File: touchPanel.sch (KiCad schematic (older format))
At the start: 41 parts, among them U11 MCP1703, U12 QT1481, U14 AFX-01_BUTTON_MATRIX, X2 16Mhz

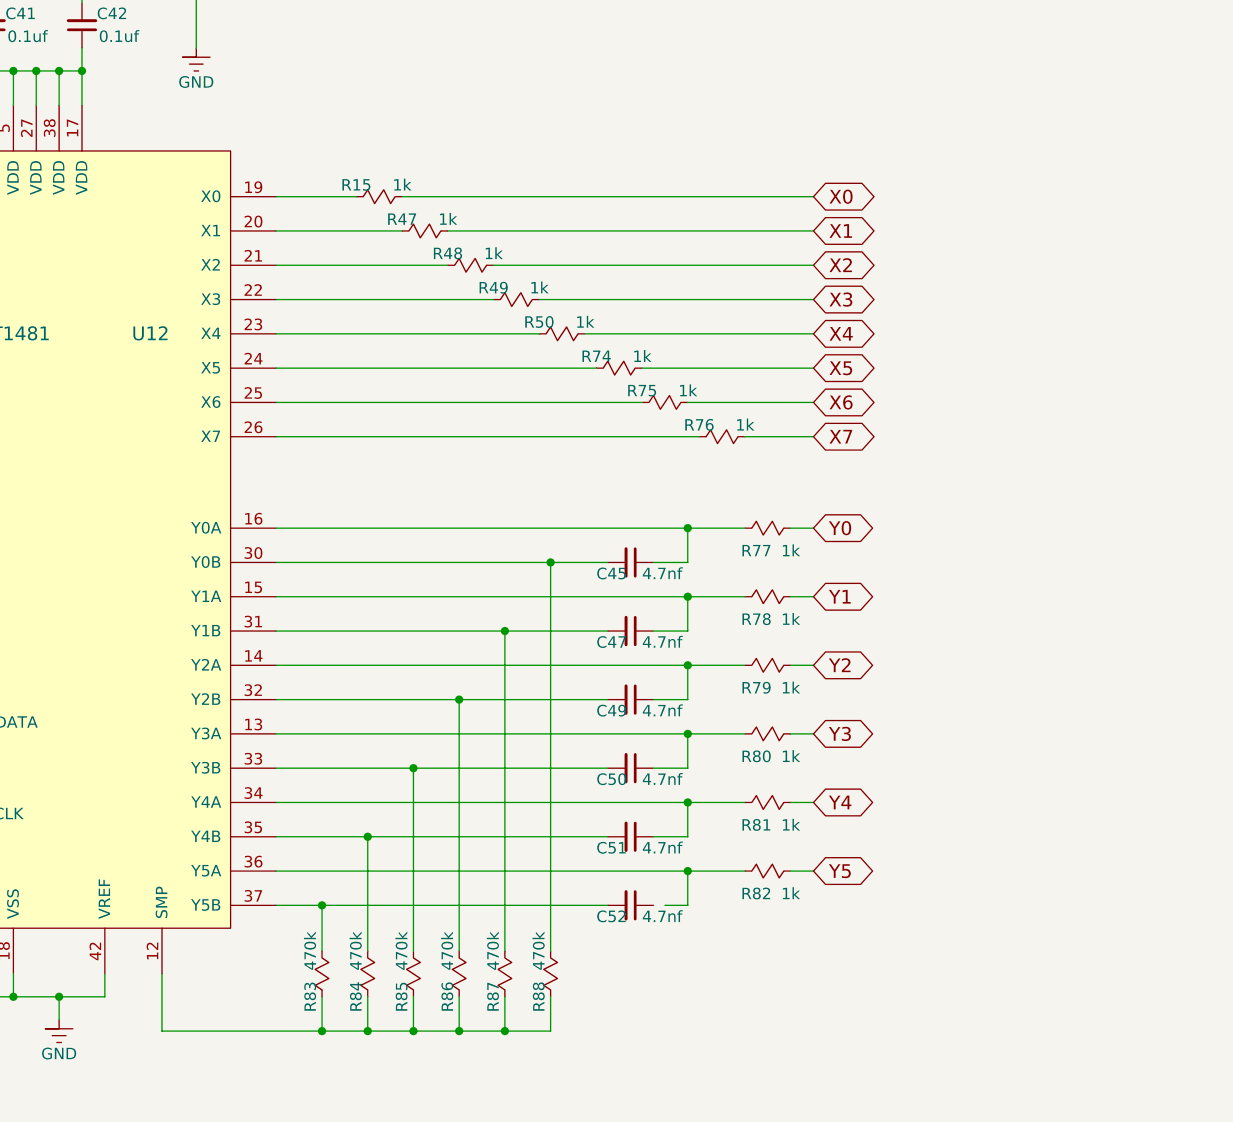
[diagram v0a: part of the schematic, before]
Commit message: Populating pcb file
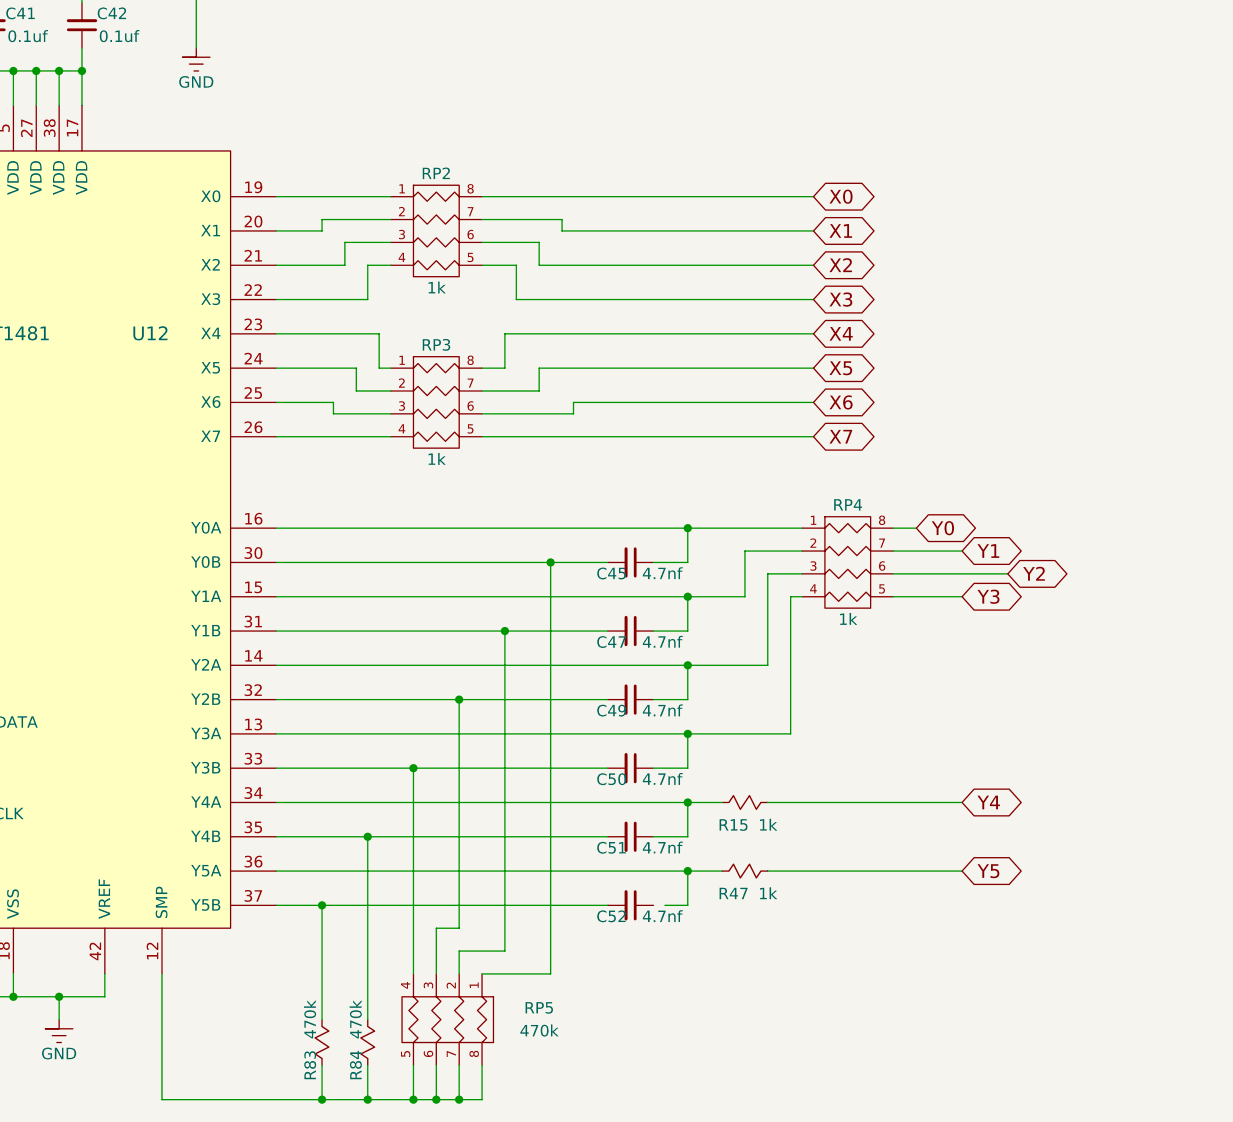
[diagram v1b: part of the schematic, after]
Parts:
- removed R48, R49, R50, R74, R75, R76, R77, R78, R79, R80, R81, R82: 1k, Resistors_SMD:R_0603_HandSoldering, symbol Resistor
- removed R85, R86, R87, R88: 470k, Resistors_SMD:R_0603_HandSoldering, symbol Resistor
- added RP2, RP3, RP4: 1k, Resistors_SMD:R_Array_Convex_4x0603, symbol R_PACK4
- added RP5: 470k, Resistors_SMD:R_Array_Convex_4x0603, symbol R_PACK4
- RP1: footprint Resistors_SMD:R_0603_HandSoldering -> Resistors_SMD:R_Array_Convex_4x0603
- U14: footprint (none) -> Zetaohm:FACEPLATEV1
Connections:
- net X0: now also RP2.8 (R1); no longer R15.1
- net X1: now also RP2.7 (R2); no longer R47.1
- net X2: now also RP2.6 (R3)
- net X3: now also RP2.5 (R4)
- net X4: now also RP3.8 (R1)
- net X5: now also RP3.7 (R2)
- net X6: now also RP3.6 (R3)
- net X7: now also RP3.5 (R4)
- net Y0: now also RP4.8 (R1)
- net Y1: now also RP4.7 (R2)
- net Y2: now also RP4.6 (R3)
- net Y3: now also RP4.5 (R4)
- net Y4: now also R15.1
- net Y5: now also R47.1
- net at R83.1, R84.1, U12.12 (SMP): now also RP5.5 (R4), RP5.6 (R3), RP5.7 (R2), RP5.8 (R1)
- net at C50.1, U12.13 (Y3A): now also RP4.4 (P4)
- net at C49.1, U12.14 (Y2A): now also RP4.3 (P3)
- net at C47.1, U12.15 (Y1A): now also RP4.2 (P2)
- net at C45.1, U12.16 (Y0A): now also RP4.1 (P1)
- net at U12.19 (X0): now also RP2.1 (P1); no longer R15.2
- net at U12.20 (X1): now also RP2.2 (P2); no longer R47.2
- net at U12.21 (X2): now also RP2.3 (P3)
- net at U12.22 (X3): now also RP2.4 (P4)
- net at U12.23 (X4): now also RP3.1 (P1)
- net at U12.24 (X5): now also RP3.2 (P2)
- net at U12.25 (X6): now also RP3.3 (P3)
- net at U12.26 (X7): now also RP3.4 (P4)
- net at C45.2, U12.30 (Y0B): now also RP5.1 (P1)
- net at C47.2, U12.31 (Y1B): now also RP5.2 (P2)
- net at C49.2, U12.32 (Y2B): now also RP5.3 (P3)
- net at C50.2, U12.33 (Y3B): now also RP5.4 (P4)
- net at C51.1, U12.34 (Y4A): now also R15.2
- net at U12.36 (Y5A): now also R47.2
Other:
- moved on the sheet: R83, R84
